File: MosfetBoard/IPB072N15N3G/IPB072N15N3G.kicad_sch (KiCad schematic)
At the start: 4 parts, among them J13 BATT+Conn2, J14 BATT-Conn2, J8 BATT+Conn1, J9 BATT-Conn1

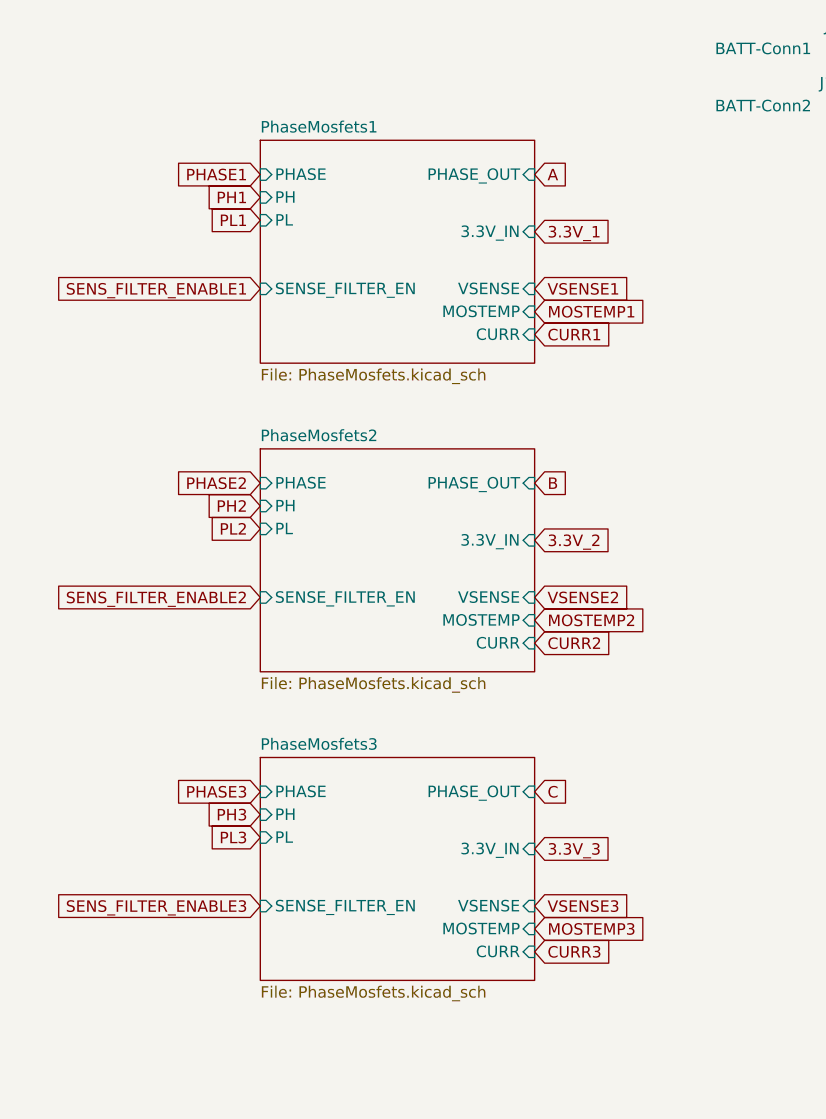
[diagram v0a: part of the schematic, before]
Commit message: cleanup
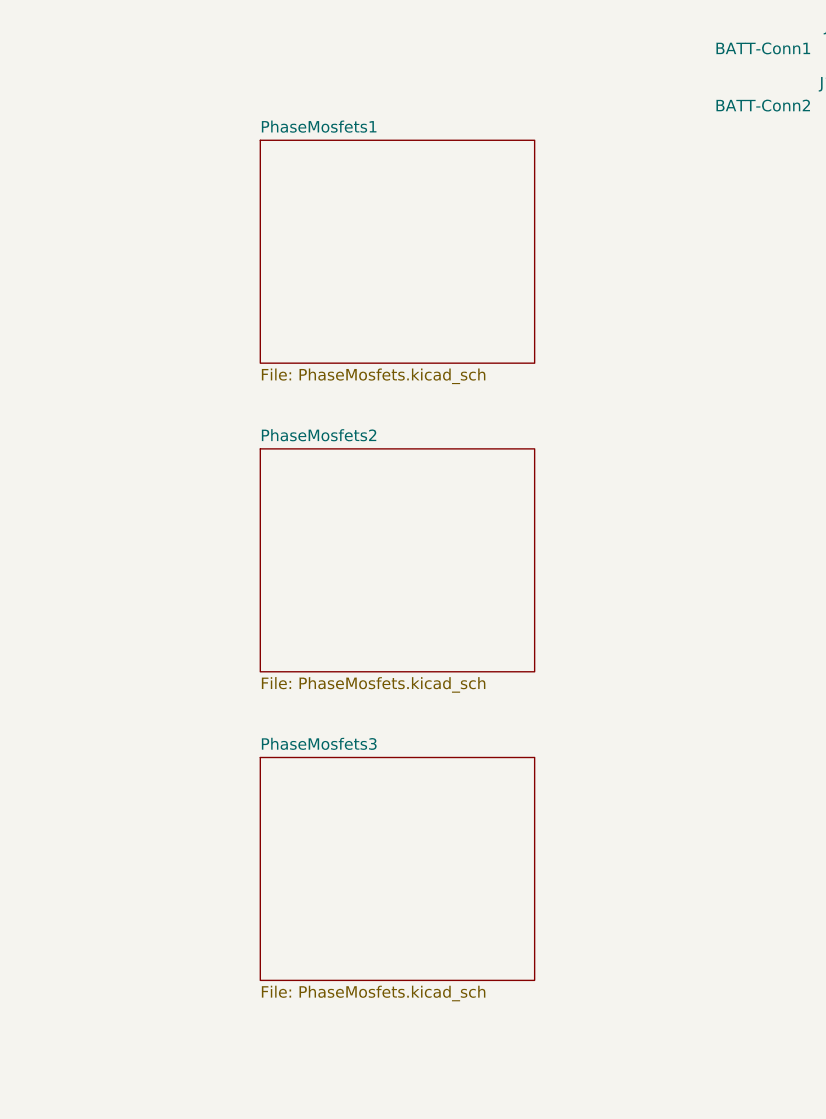
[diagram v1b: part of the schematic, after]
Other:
- sheet PhaseMosfets1 ports: added none; removed 3.3V_IN, CURR, MOSTEMP, PH, PHASE, PHASE_OUT, PL, SENSE_FILTER_EN, VSENSE
- sheet PhaseMosfets2 ports: added none; removed 3.3V_IN, CURR, MOSTEMP, PH, PHASE, PHASE_OUT, PL, SENSE_FILTER_EN, VSENSE
- sheet PhaseMosfets3 ports: added none; removed 3.3V_IN, CURR, MOSTEMP, PH, PHASE, PHASE_OUT, PL, SENSE_FILTER_EN, VSENSE

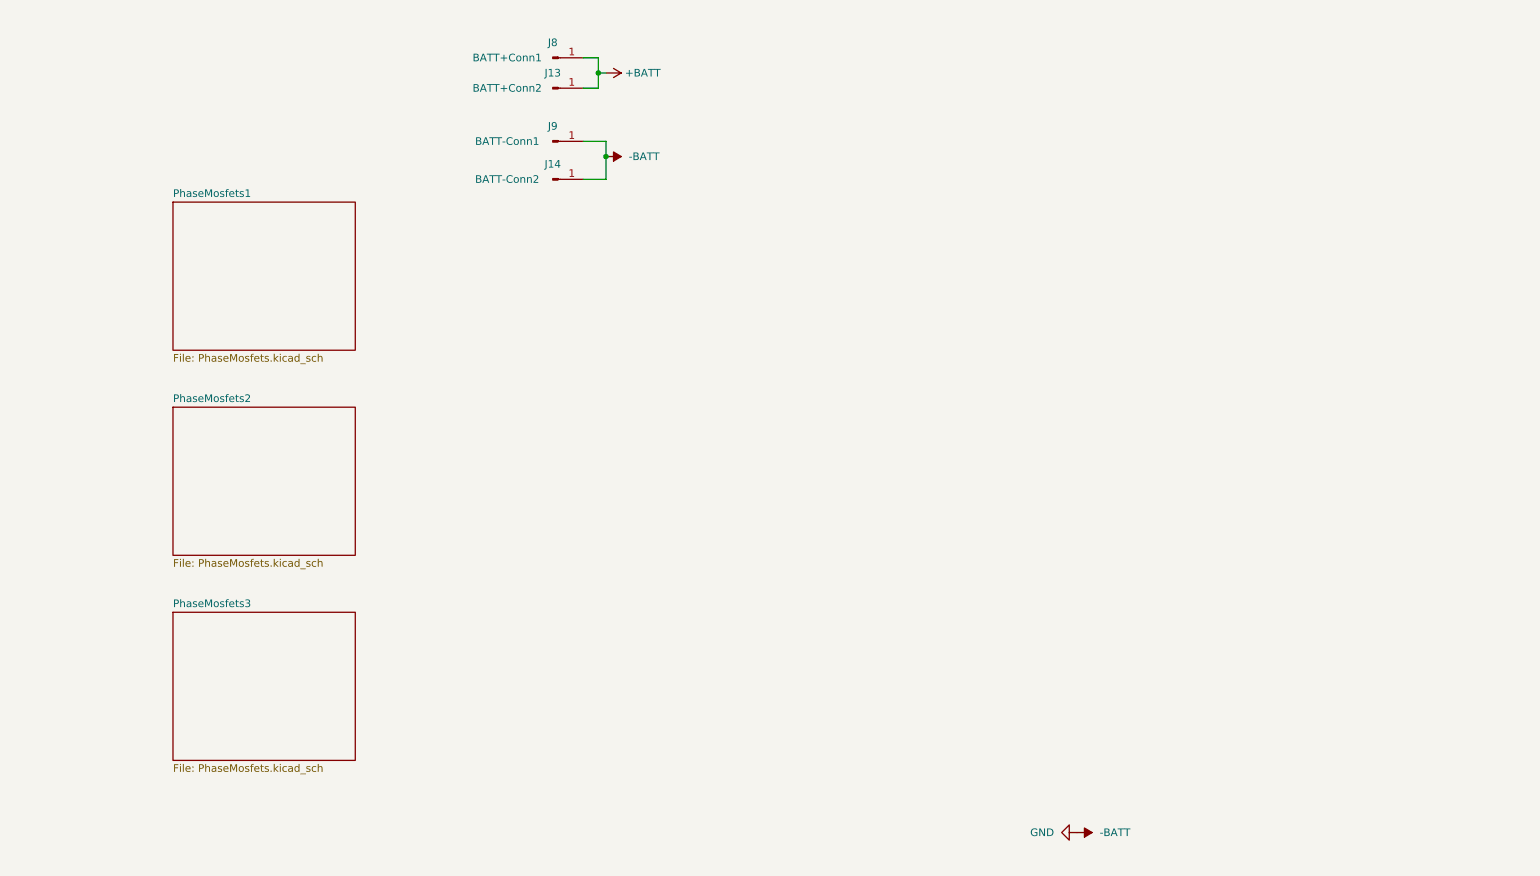
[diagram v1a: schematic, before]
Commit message: v3.0.2 - IPB v2
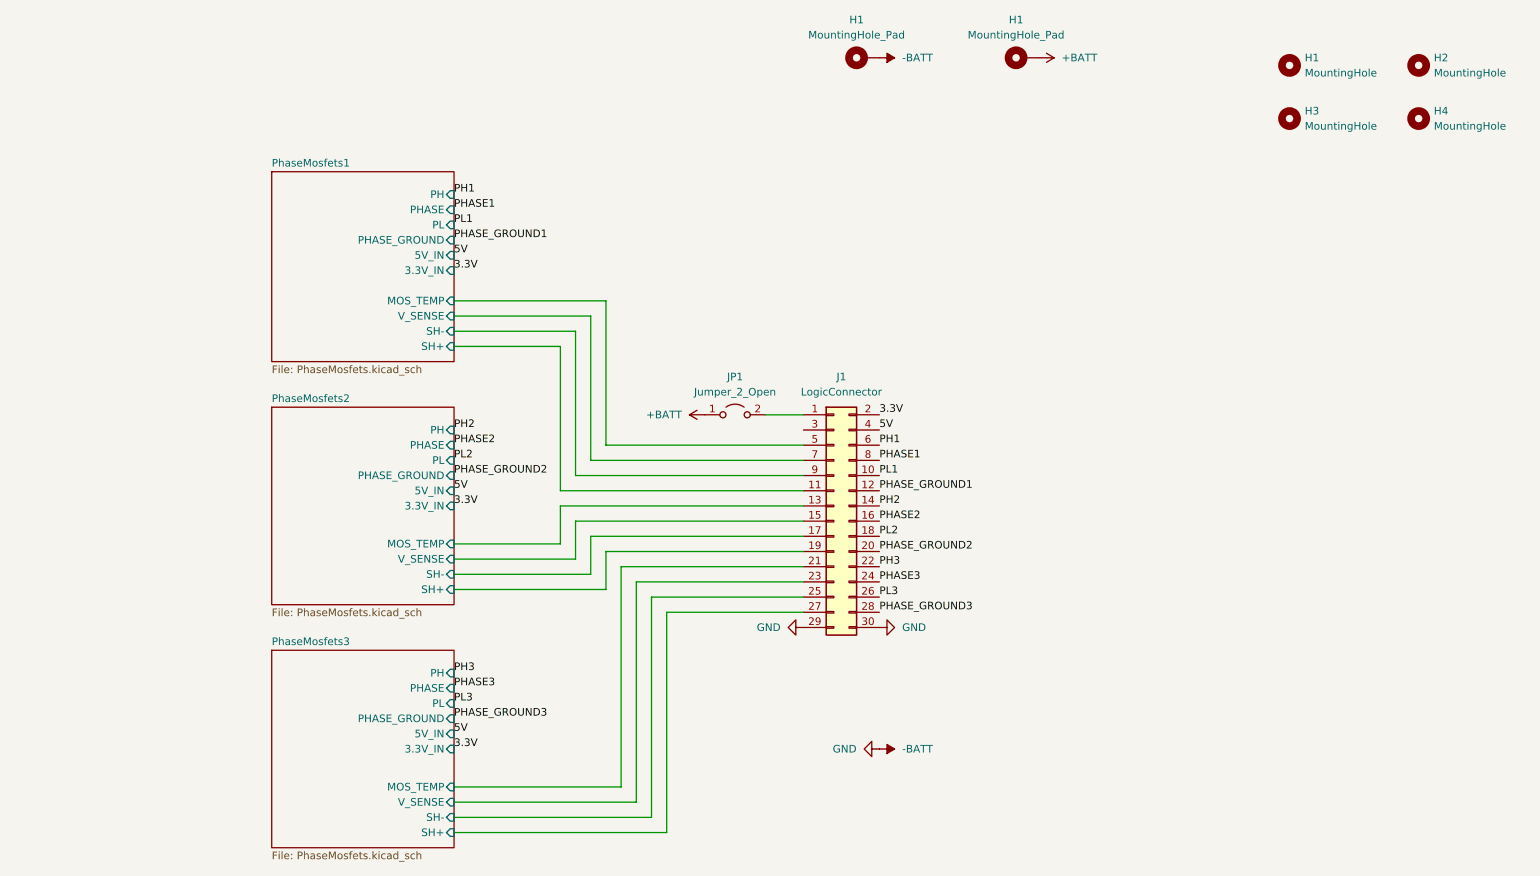
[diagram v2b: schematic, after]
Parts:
- removed J13: BATT+Conn2, Connector_Wire:SolderWirePad_1x01_SMD_5x10mm, symbol Connector:Conn_01x01_Pin
- removed J14: BATT-Conn2, Connector_Wire:SolderWirePad_1x01_SMD_5x10mm, symbol Connector:Conn_01x01_Pin
- removed J8: BATT+Conn1, Connector_Wire:SolderWirePad_1x01_SMD_5x10mm, symbol Connector:Conn_01x01_Pin
- removed J9: BATT-Conn1, Connector_Wire:SolderWirePad_1x01_SMD_5x10mm, symbol Connector:Conn_01x01_Pin
- added H1 (x2): MountingHole_Pad, MountingHole:MountingHole_5.3mm_M5_Pad_Via, symbol Mechanical:MountingHole_Pad
- added H1, H2, H3, H4: MountingHole, MountingHole:MountingHole_3.2mm_M3_ISO14580, symbol Mechanical:MountingHole
- added J1: LogicConnector, Connector_PinSocket_2.54mm:PinSocket_2x15_P2.54mm_Vertical, symbol Connector_Generic:Conn_02x15_Odd_Even
- added JP1: Jumper_2_Open, GigaVescLibs:SolderJumper0.5mm_Open, symbol Jumper:Jumper_2_Open
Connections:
- net +BATT: now also H1.1, JP1.1 (A)
- net -BATT: now also H1.1, J1.29 (Pin_29), J1.30 (Pin_30)
- new net: J1.1 (Pin_1), JP1.2 (B)
- new net 3.3V: J1.2 (Pin_2)
- new net 5V: J1.4 (Pin_4)
- new net PH1: J1.6 (Pin_6)
- new net PH2: J1.14 (Pin_14)
- new net PH3: J1.22 (Pin_22)
- new net PHASE1: J1.8 (Pin_8)
- new net PHASE2: J1.16 (Pin_16)
- new net PHASE3: J1.24 (Pin_24)
- new net PHASE_GROUND1: J1.12 (Pin_12)
- new net PHASE_GROUND2: J1.20 (Pin_20)
- new net PHASE_GROUND3: J1.28 (Pin_28)
- new net PL1: J1.10 (Pin_10)
- new net PL2: J1.18 (Pin_18)
- new net PL3: J1.26 (Pin_26)
- new net PhaseMosfets1/MOS_TEMP: J1.5 (Pin_5)
- new net PhaseMosfets1/SH+: J1.11 (Pin_11)
- new net PhaseMosfets1/SH-: J1.9 (Pin_9)
- new net PhaseMosfets1/V_SENSE: J1.7 (Pin_7)
- new net PhaseMosfets2/MOS_TEMP: J1.13 (Pin_13)
- new net PhaseMosfets2/SH+: J1.19 (Pin_19)
- new net PhaseMosfets2/SH-: J1.17 (Pin_17)
- new net PhaseMosfets2/V_SENSE: J1.15 (Pin_15)
- new net PhaseMosfets3/MOS_TEMP: J1.21 (Pin_21)
- new net PhaseMosfets3/SH+: J1.27 (Pin_27)
- new net PhaseMosfets3/SH-: J1.25 (Pin_25)
- new net PhaseMosfets3/V_SENSE: J1.23 (Pin_23)
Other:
- sheet PhaseMosfets1 ports: added 3.3V_IN, 5V_IN, MOS_TEMP, PH, PHASE, PHASE_GROUND, PL, SH+, SH-, V_SENSE; removed none
- sheet PhaseMosfets2 ports: added 3.3V_IN, 5V_IN, MOS_TEMP, PH, PHASE, PHASE_GROUND, PL, SH+, SH-, V_SENSE; removed none
- sheet PhaseMosfets3 ports: added 3.3V_IN, 5V_IN, MOS_TEMP, PH, PHASE, PHASE_GROUND, PL, SH+, SH-, V_SENSE; removed none
